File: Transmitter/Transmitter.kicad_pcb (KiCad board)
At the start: 2 copper layers, 106.7 x 88.9 mm, 18 parts, among them IC1 TORX1950A_F_, IC2 TORX1950A_F_, IC3 TORX1950A_F_, J1 Conn_01x08_Male

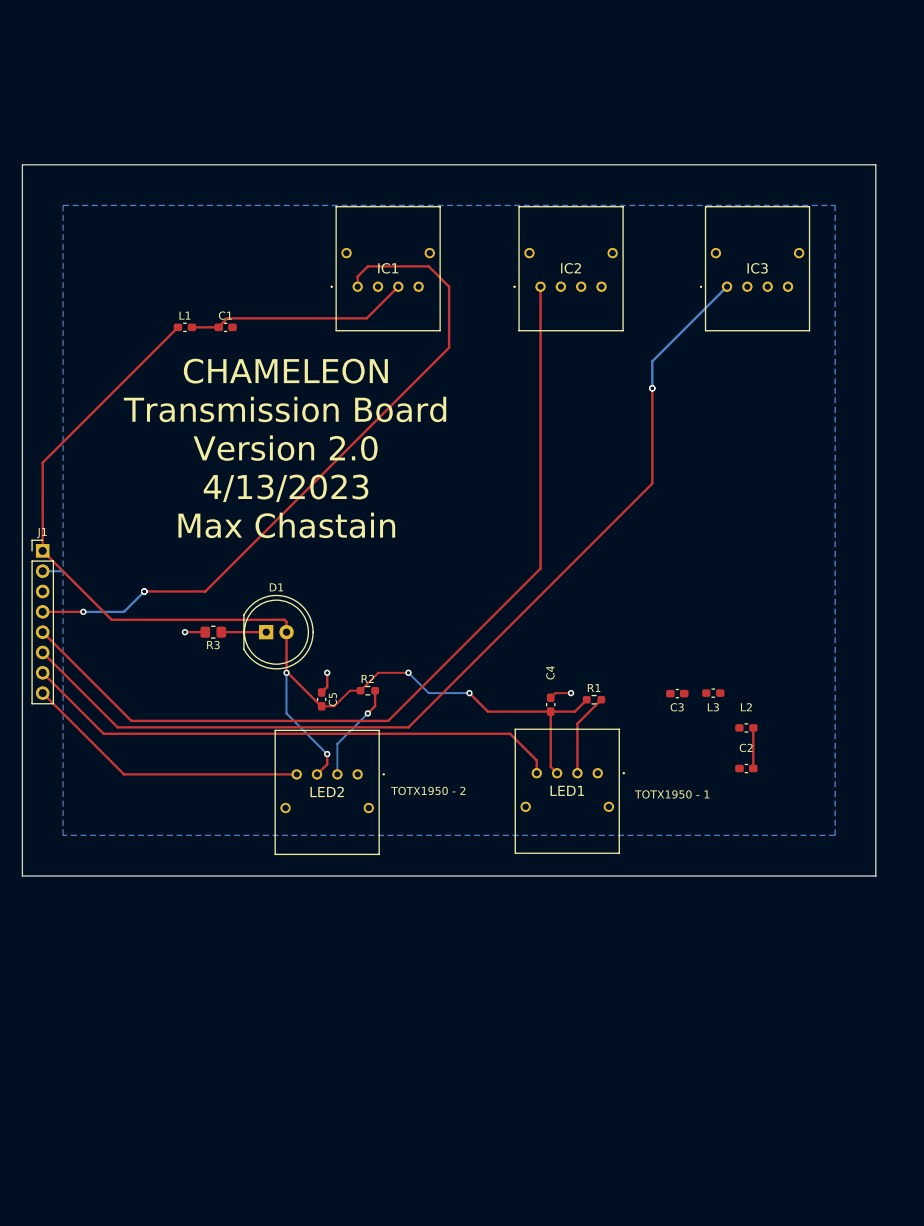
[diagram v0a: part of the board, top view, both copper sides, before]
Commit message: Version 3 transmitter
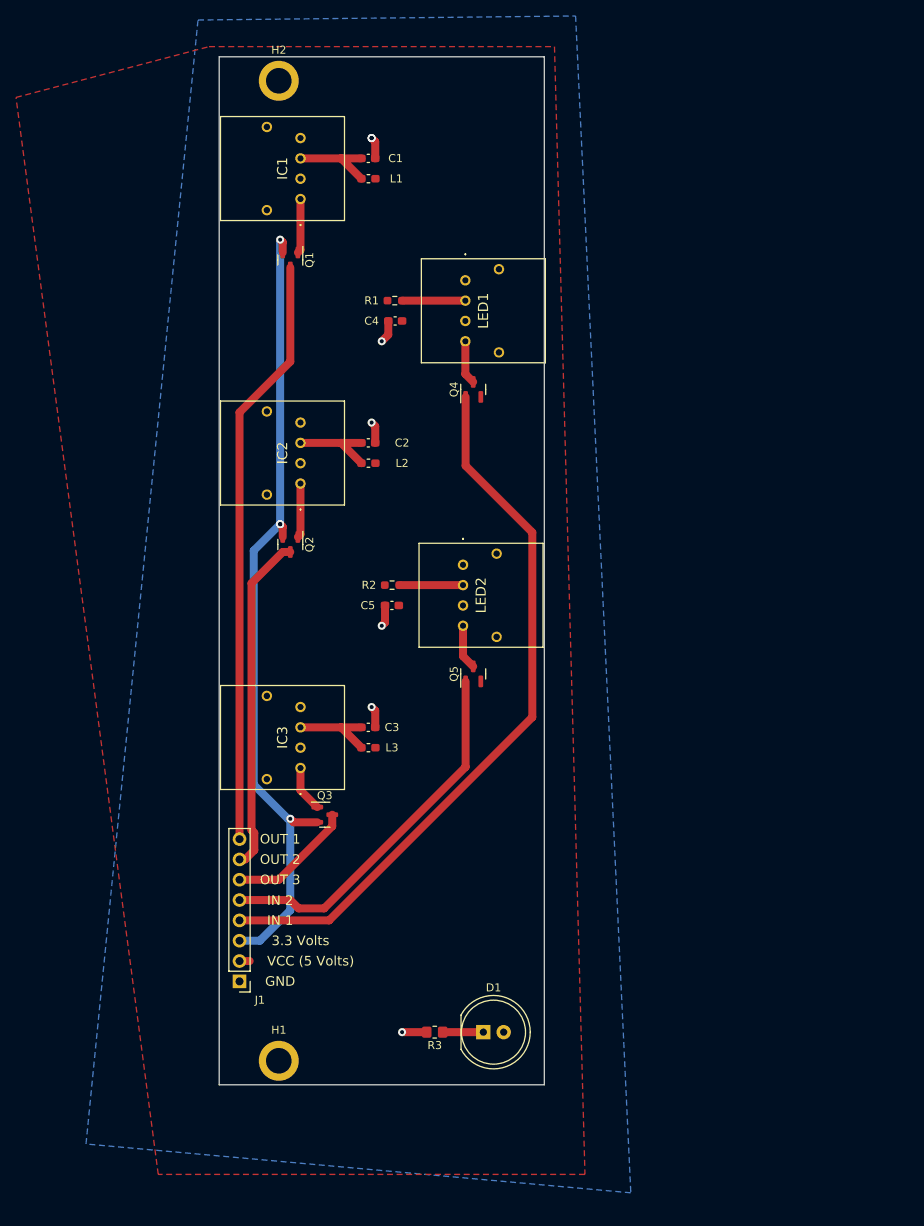
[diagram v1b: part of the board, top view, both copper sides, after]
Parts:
- added H1: MountingHole_Pad, MountingHole:MountingHole_3.2mm_M3_ISO7380_Pad, F.Cu at (57.5, 175.5)
- added H2: MountingHole_Pad, MountingHole:MountingHole_3.2mm_M3_ISO7380_Pad, F.Cu at (57.5, 53.0)
- added Q1: BSS138, Package_TO_SOT_SMD:SOT-23, F.Cu at (58.9, 75.4)
- added Q2: BSS138, Package_TO_SOT_SMD:SOT-23, F.Cu at (58.9, 111.0)
- added Q3: BSS138, Package_TO_SOT_SMD:SOT-23, F.Cu at (63.2, 144.7)
- added Q4: BSS138, Package_TO_SOT_SMD:SOT-23, F.Cu at (81.8, 91.6)
- added Q5: BSS138, Package_TO_SOT_SMD:SOT-23, F.Cu at (81.8, 127.1)
- IC1, IC2, IC3: footprint KiCad:TORX1950AF -> TOTX and TORX:TORX1950AF
- LED1, LED2: footprint KiCad:TOTX1950AF -> TOTX and TORX:TOTX1950AF
- R3: value 1.5k -> 10k
- moved IC3 80.4 mm to (60.2, 138.9), turned to 90 degrees
- moved C2 62.4 mm to (68.6, 98.3), turned to 0 degrees
- moved J1 59.2 mm to (52.5, 165.6), turned to 180 degrees
- moved L2 57.7 mm to (68.7, 100.8), turned to 180 degrees
- moved R3 57.2 mm to (76.9, 171.9)
- moved D1 56.9 mm to (83.0, 171.9)
- moved LED1 56.5 mm to (80.8, 85.6), turned to -90 degrees
- moved R1 55.8 mm to (71.9, 80.5)
- moved C4 51.8 mm to (72.0, 83.0), turned to 0 degrees
- moved L3 43.6 mm to (68.7, 136.4)
- moved C3 38.9 mm to (68.6, 133.8), turned to 0 degrees
- moved IC2 38.8 mm to (60.2, 103.3), turned to 90 degrees
- moved L1 29.5 mm to (68.7, 65.2), turned to 180 degrees
- moved C1 27.6 mm to (68.6, 62.7)
- moved LED2 22.8 mm to (80.5, 121.1), turned to -90 degrees
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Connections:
- IC1 pad 1: OUT1 -> Net-(IC1-Pad1)
- IC2 pad 1: OUT2 -> Net-(IC2-Pad1)
- IC3 pad 1: OUT3 -> Net-(IC3-Pad1)
- J1 pad 1: VCC -> GND
- J1 pad 2: GND -> VCC
- J1 pad 3: unconnected-(J1-Pad3) -> +3.3V
- J1 pad 4: OUT1 -> /IN 1
- J1 pad 5: OUT2 -> /IN 2
- J1 pad 6: OUT3 -> /OUT 3
- J1 pad 7: IN1 -> /OUT 2
- J1 pad 8: IN2 -> /OUT 1
- LED1 pad 4: IN1 -> Net-(LED1-Pad4)
- LED2 pad 4: IN2 -> Net-(LED2-Pad4)
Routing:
- net VCC: track 142.4 -> 1.27 mm, vias 4 -> 0
- net OUT3: track 121.2 -> 0.00 mm, vias 2 -> 0
- net OUT2: track 109.9 -> 0.00 mm
- net +3.3V: track 0.00 -> 102.2 mm, vias 0 -> 4
- net /IN 1: track 0.00 -> 90.6 mm
- net OUT1: track 86.4 -> 0.00 mm, vias 4 -> 0
- net /OUT 1: track 0.00 -> 74.1 mm
- net IN1: track 67.9 -> 0.00 mm
- net /IN 2: track 0.00 -> 46.7 mm
- net /OUT 2: track 0.00 -> 42.3 mm
- net IN2: track 36.0 -> 0.00 mm
- net Net-(C1-Pad1): track 27.9 -> 11.2 mm
- net /OUT 3: track 0.00 -> 15.8 mm
- net Net-(C3-Pad1): track 0.08 -> 11.2 mm
- net Net-(IC1-Pad1): track 0.00 -> 6.82 mm
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- added copper zone on F.Cu, net VCC
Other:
- board size 106.7 x 88.9 mm -> 40.6 x 128.5 mm
- board text added: "3.3 Volts"
- board text added: "GND"
- board text added: "IN 1"
- board text added: "IN 2"
- board text added: "OUT 1"
- board text added: "OUT 2"
- board text added: "OUT 3"
- board text added: "VCC (5 Volts)"
- board text removed: "CHAMELEON Transmission Board Version 2.0 4/13/2023 Max Chastain"
- board text removed: "TOTX1950 - 1"
- board text removed: "TOTX1950 - 2"
